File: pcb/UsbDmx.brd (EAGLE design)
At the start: 24 parts, among them IC4 SN75176ASOIC, J1 RS485, J2 POWER_JACKPTH, Q1 16MHz 10ppm, X1 USBPTH

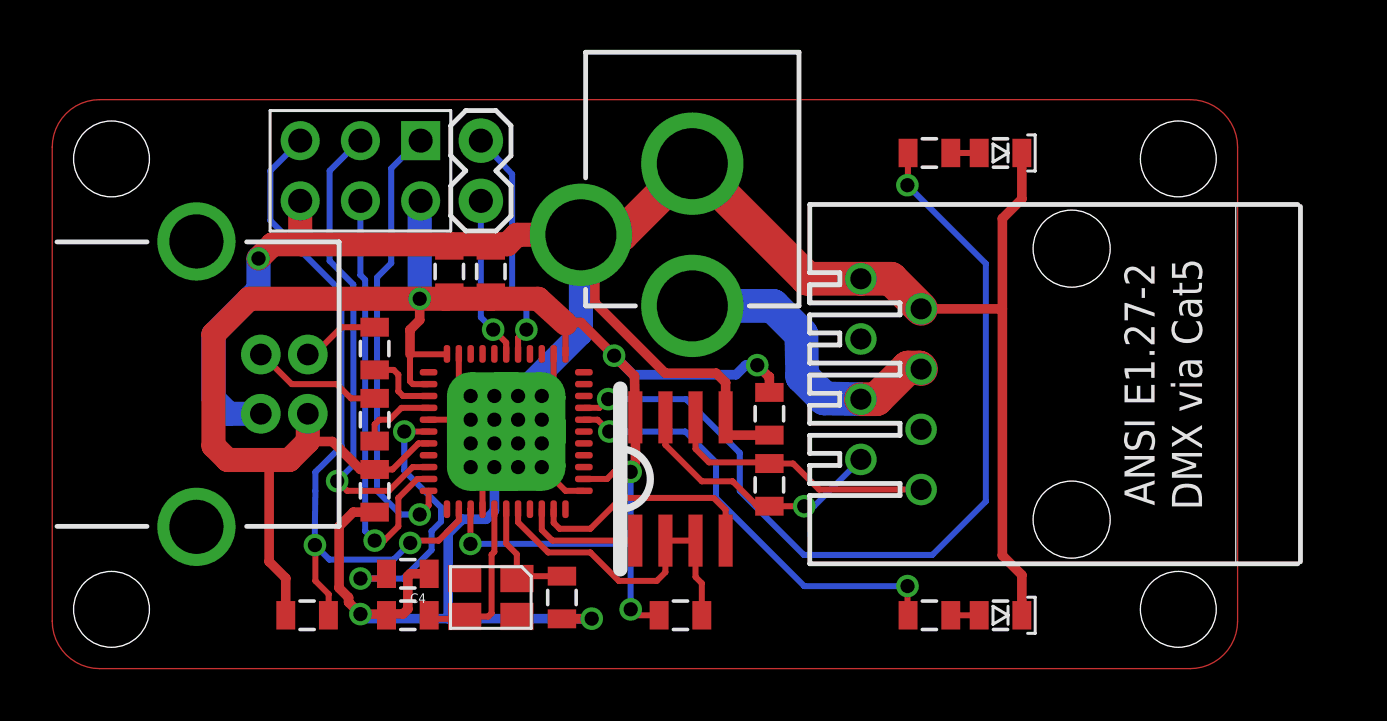
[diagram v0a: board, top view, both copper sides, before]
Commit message: RevB, as submitted
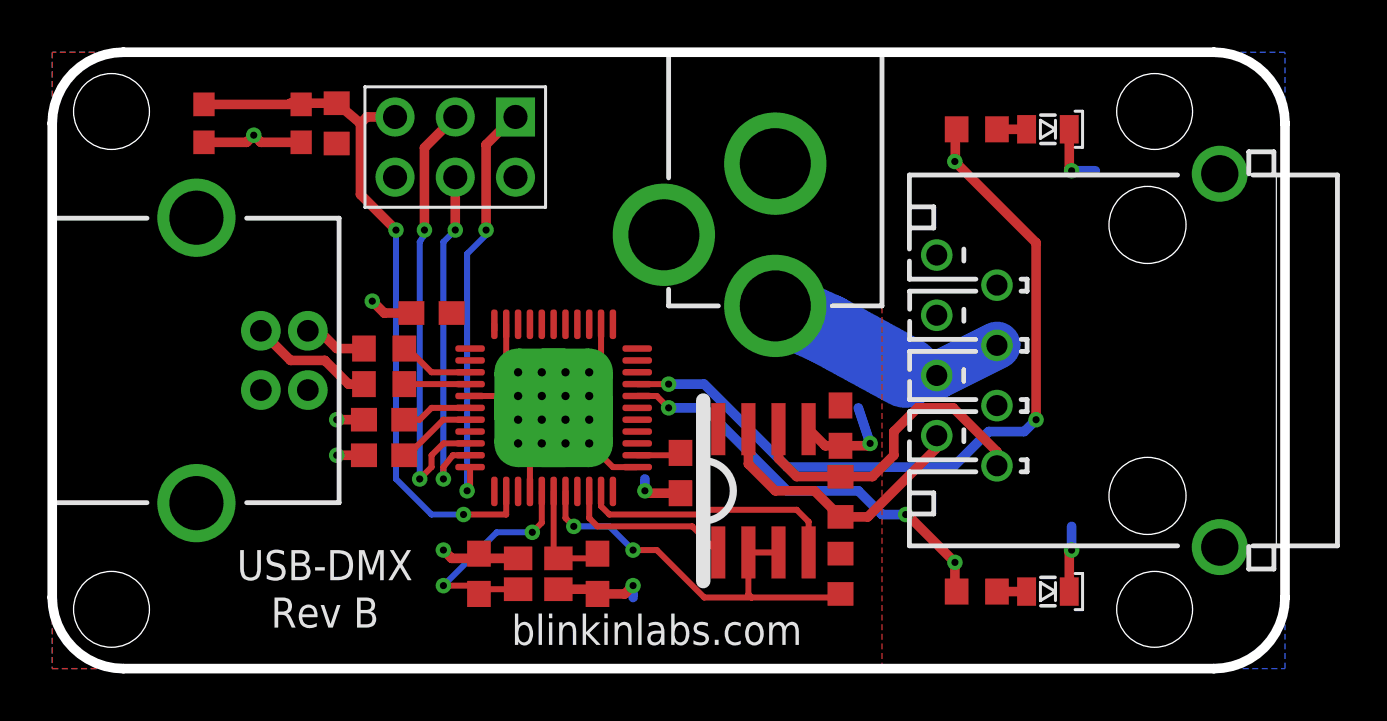
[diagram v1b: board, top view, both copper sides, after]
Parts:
- removed J1: RS485, con-amp:520426-4
- removed JP1: (no value), SparkFun:1X02
- added J3: (no value), con-amp:555153-1
- added U$3: (no value), blinkinlabs:BUTTON_MOMENTARY_KMR211G
- C1, C2, C4, C5, C6, C7: device SparkFun:0805 -> adafruit:C0603
- C3: value .1uF -> 100nF; device SparkFun:0805 -> adafruit:C0603
- Q1: device blinkyboard:XS3225 -> blinkinlabs:CRSYTAL_2520
- R1, R2, R3, R4, R5, R6, R8: device SparkFun:0805 -> adafruit:R0603
- U$1: value ARDUINO_LEONARDO-REV3B_SMARTPRJ_ATMEGA32U4-XUMU -> ARDUINO_LEONARDO-REV3B_SMARTPRJ_ATMEGA32U4-XUMU_LONG; device blinkinlabs:ARDUINO_LEONARDO-REV3B_SMARTPRJ_QFN44ML7X7 -> blinkinlabs:QFN44ML7X7_LONGLEADS
- moved R4 20.8 mm to (12.0, 23.0), turned to 270 degrees
- moved C7 11.7 mm to (26.5, 8.25)
- moved R2 6.97 mm to (33.2, 4.00), turned to 90 degrees
- moved C4 6.58 mm to (14.0, 10.5)
- moved U$2 4.12 mm to (17.0, 22.0)
- moved IC4 3.54 mm to (30.0, 7.50)
- moved J2 3.50 mm to (30.5, 29.0)
- moved C1 3.47 mm to (18.0, 4.00), turned to 90 degrees
- moved C5 3.04 mm to (33.2, 10.2), turned to 270 degrees
- moved R1 3.04 mm to (33.2, 7.25)
- moved DEBUG 2.24 mm to (42.0, 3.25)
- moved DEBUG1 2.24 mm to (42.0, 22.8)
- moved Q1 2.24 mm to (20.5, 4.00)
- moved R3 2.24 mm to (39.0, 22.8)
- moved R8 2.24 mm to (39.0, 3.25)
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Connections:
- removed net A2: JP1.2, U$1.38
- removed net A3: JP1.1, U$1.39
- new net RXLED: U$1.8
- new net TXLED: U$1.22
- net GND: now also C1.2, C2.2, C3.2, C4.2, C5.2, C6.2, C7.2, J3.7, J3.8, Q1.P$2, Q1.P$4, U$3.P$1, U$3.P$2; no longer C1.1, C2.1, C3.1, C4.1, C5.1, C6.1, C7.1, J1.7, J1.8
- net N$2: now also C1.1; no longer C1.2
- net N$5: now also C2.1; no longer C2.2
- net N$9: now also C4.1; no longer C4.2
- net RESET: now also U$3.P$3, U$3.P$4
- net RS485A: now also J3.1; no longer J1.1
- net RS485B: now also J3.2; no longer J1.2
- net VCC: now also C3.1, C5.1, C6.1, C7.1; no longer C3.2, C5.2, C6.2, C7.2
- net VMOT: now also J3.4, J3.5; no longer J1.4, J1.5
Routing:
- net N$11: track 143.3 -> 0.00 mm
- net GND: track 143.1 -> 42.6 mm, vias 3 -> 10
- net VCC: track 85.2 -> 5.58 mm, vias 6 -> 0
- net A2: track 9.94 -> 0.00 mm, vias 1 -> 0
- net N$9: track 11.6 -> 2.98 mm, vias 2 -> 0
- net A3: track 6.90 -> 0.00 mm, vias 1 -> 0
- net D10: track 37.8 -> 32.8 mm, vias 2 -> 3
- net MOSI: track 18.6 -> 14.8 mm, vias 1 -> 2
- net D3: track 13.8 -> 17.4 mm, vias 0 -> 2
- net N$2: track 7.23 -> 10.1 mm, vias 0 -> 2
- net RX: track 5.01 -> 7.61 mm
- net RS485A: track 11.5 -> 13.9 mm
- net VMOT: track 12.9 -> 10.6 mm
- net RESET: track 30.0 -> 31.3 mm
- net MISO: track 18.9 -> 17.7 mm, vias 1 -> 2
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- added copper zone on layer 16, net GND
- added copper zone on layer 1, net VCC
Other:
- board outline added: 52 x 26 mm
- board text added: "Rev B"
- board text removed: "ANSI E1.27-2"
- board text removed: "DMX via Cat5"
- board text removed: "Rev A"
